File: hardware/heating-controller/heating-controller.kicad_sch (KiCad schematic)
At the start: 22 parts, among them J1 LilyGo T-Display S3, J2 Temperature_probes, J3 Power connector, K1 FINDER-32.21-x000, Q1 AO3400A, U1 H11AA1

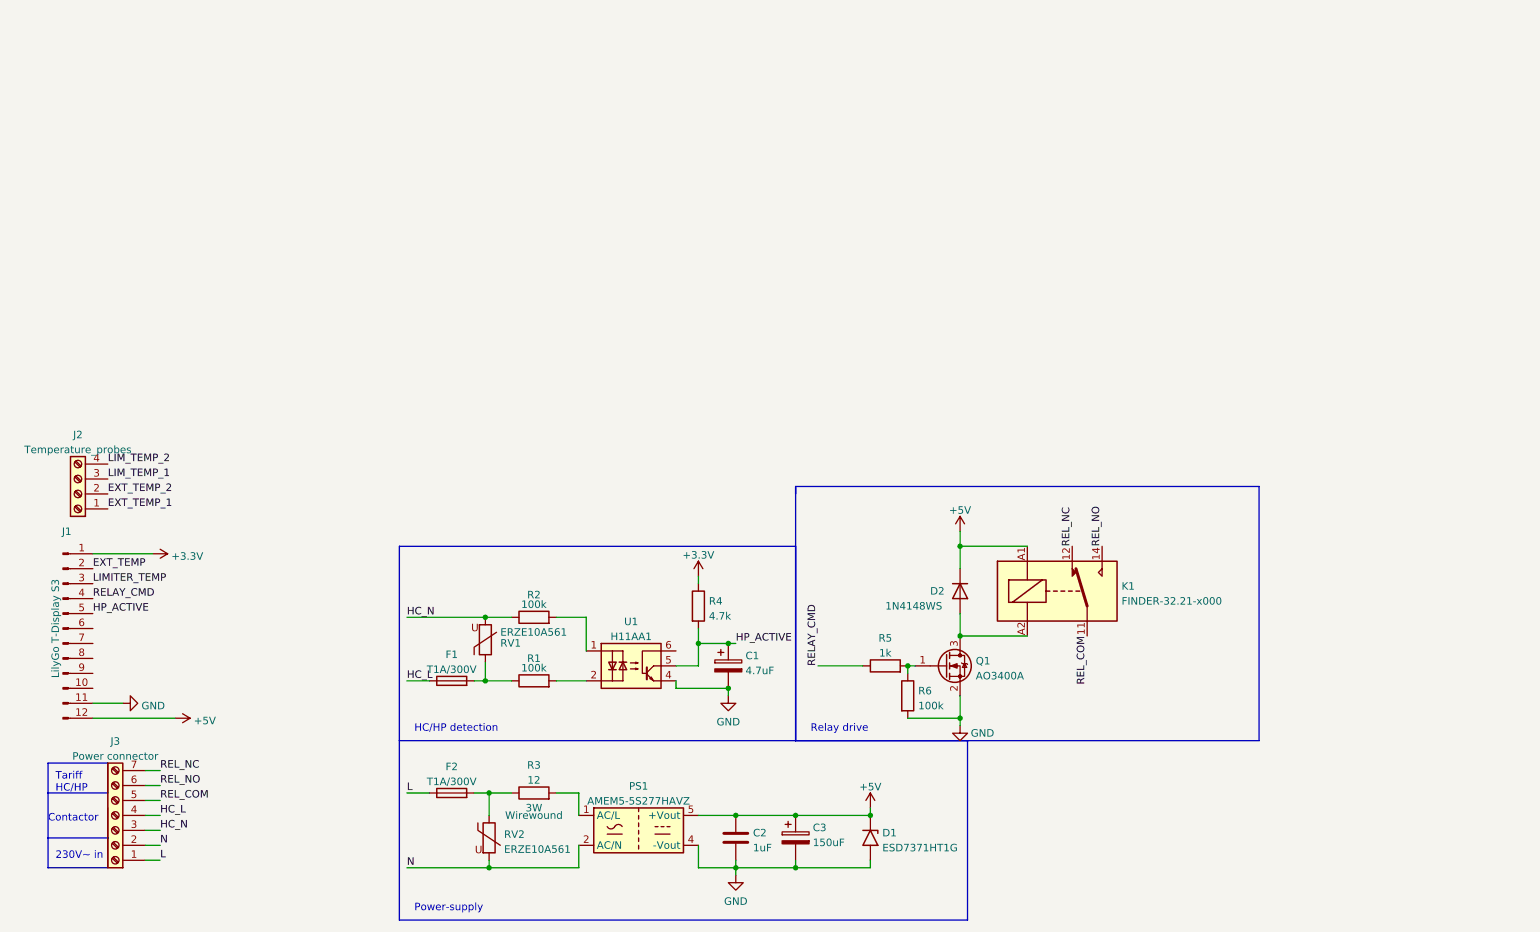
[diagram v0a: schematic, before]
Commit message: First PCB, needs to be checked
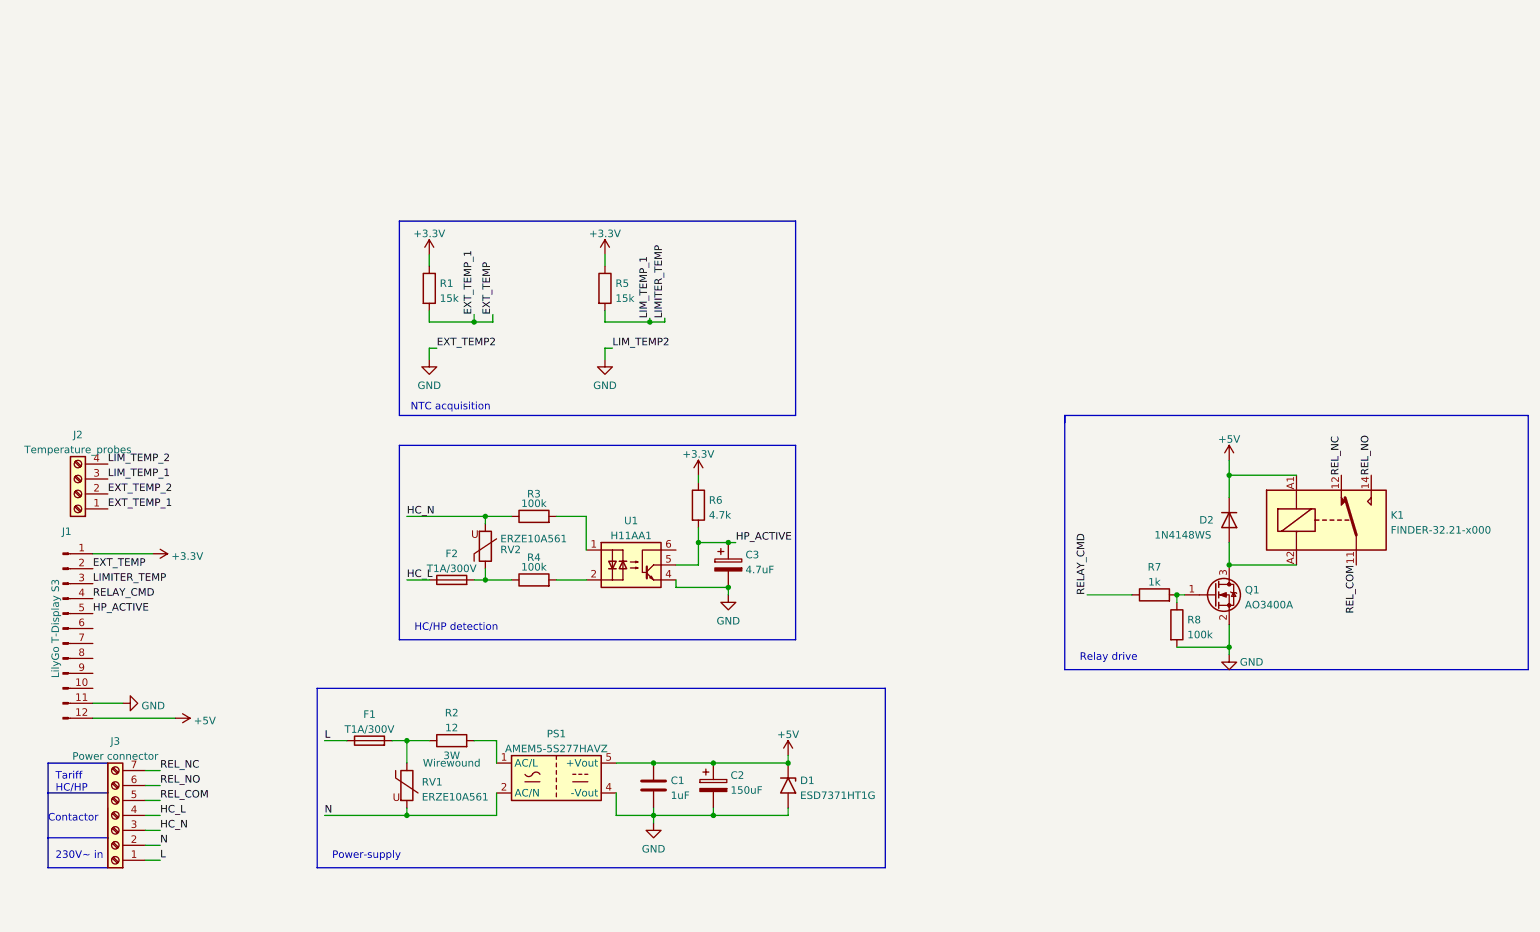
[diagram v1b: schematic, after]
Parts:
- added R1, R5: 15k, Resistor_SMD:R_0603_1608Metric, symbol Device:R
- C1: renamed from C2; footprint Resistor_SMD:R_0201_0603Metric -> Capacitor_SMD:C_0603_1608Metric
- renumbered C3 to C2, C1 to C3, F2 to F1, F1 to F2, R3 to R2, R2 to R3, R1 to R4, R4 to R6, R5 to R7, R6 to R8, RV2 to RV1, RV1 to RV2
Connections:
- net EXT_TEMP_1 is gone; now on net EXT_TEMP: J2.1 (Pin_1)
- net LIM_TEMP_1 is gone; now on net LIMITER_TEMP: J2.3 (Pin_3)
- net +3.3V: now also R1.1, R5.1
- net EXT_TEMP: now also R1.2
- net LIMITER_TEMP: now also R5.2
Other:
- note added: "NTC acquisition"
- moved on the sheet: C1, C2, C3, D1, D2, F1, F2, K1, PS1, Q1, R2, R3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

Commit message: WIP
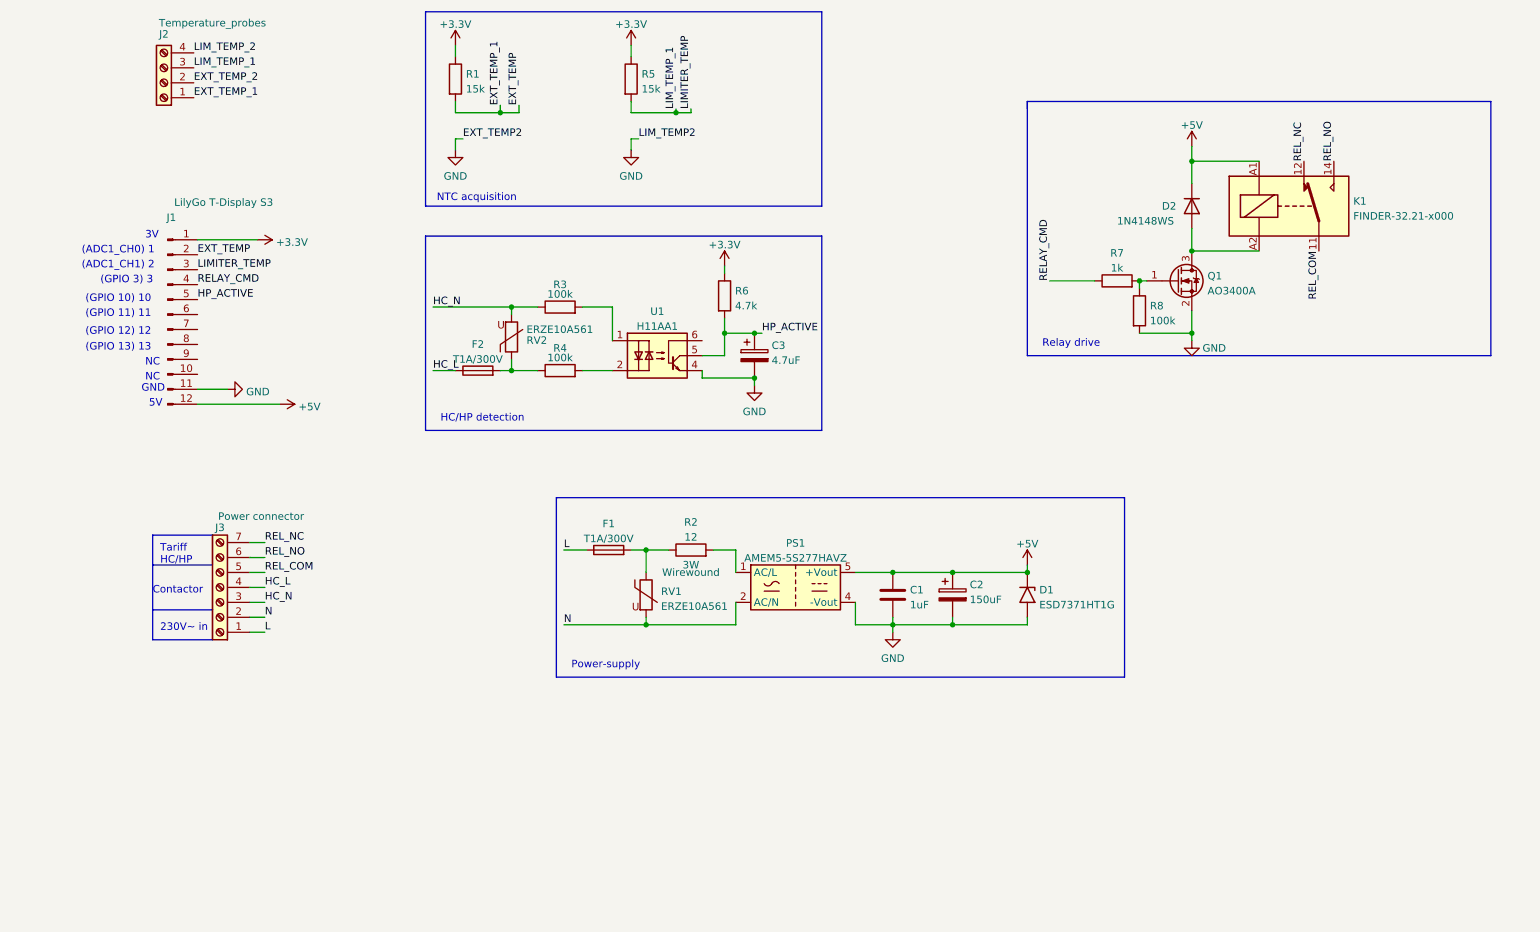
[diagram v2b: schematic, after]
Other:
- note added: "(ADC1_CH0) 1"
- note added: "(ADC1_CH1) 2"
- note added: "(GPIO 10) 10"
- note added: "(GPIO 11) 11"
- note added: "(GPIO 12) 12"
- note added: "(GPIO 13) 13"
- note added: "(GPIO 3) 3"
- note added: "3V"
- note added: "5V"
- note added: "GND"
- note added: "NC"
- moved on the sheet: C1, C2, C3, D1, D2, F1, F2, J1, J2, J3, K1, PS1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
